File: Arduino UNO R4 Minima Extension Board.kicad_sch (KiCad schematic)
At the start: 11 parts, among them J1 Power, J2 Analog, J3 Digital/PWM, J4 Digital/PWM, J5 Conn_01x04_Socket, J6 Conn_01x04_Socket, J7 Conn_01x05_Socket, J8 Conn_01x05_Socket, J9 Conn_01x05_Socket, U1 MCP2551-I-SN

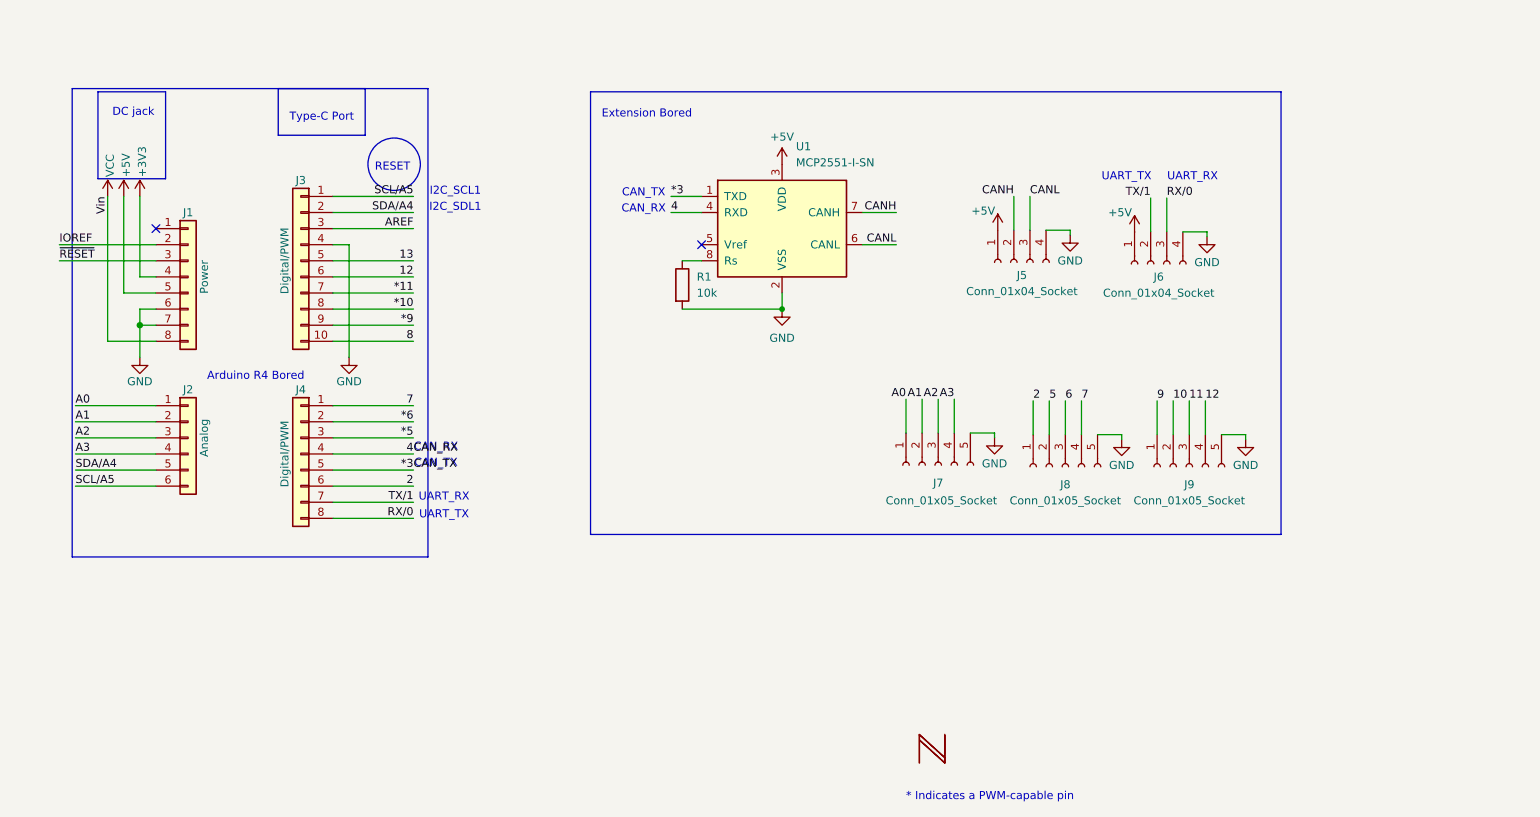
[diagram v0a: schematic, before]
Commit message: Add files via upload
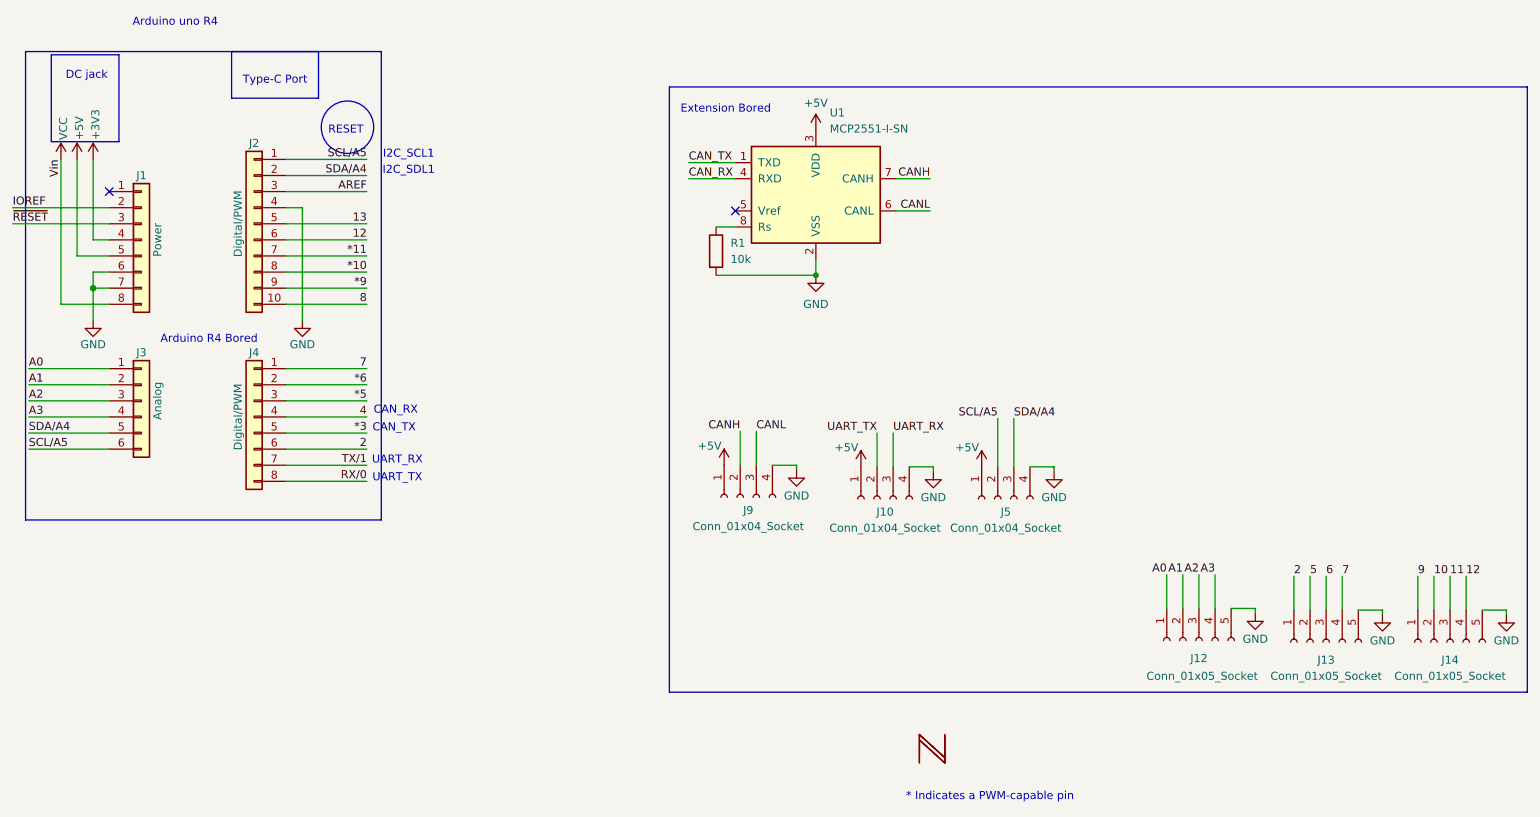
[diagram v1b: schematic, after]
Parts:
- added J5: Conn_01x04_Socket, Connector_JST:JST_XA_S04B-XASK-1_1x04_P2.50mm_Horizontal, symbol Connector:Conn_01x04_Socket
- renumbered J6 to J10, J7 to J12, J8 to J13, J9 to J14, J3 to J2, J2 to J3, J5 to J9
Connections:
- net *3: no longer U1.1 (TXD)
- net +5V: now also J5.1 (Pin_1)
- net 4: no longer U1.4 (RXD)
- net GND: now also J5.4 (Pin_4)
- net RX/0: no longer J10.3 (Pin_3)
- net SCL/A5: now also J5.2 (Pin_2)
- net SDA/A4: now also J5.3 (Pin_3)
- net TX/1: no longer J10.2 (Pin_2)
- new net CAN_RX: U1.4 (RXD)
- new net CAN_TX: U1.1 (TXD)
- new net UART_RX: J10.3 (Pin_3)
- new net UART_TX: J10.2 (Pin_2)
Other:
- note added: "Arduino uno R4"
- moved on the sheet: J1, J10, J12, J13, J14, J2, J3, J4, J9, R1, U1
